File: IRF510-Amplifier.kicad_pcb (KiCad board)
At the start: 2 copper layers, 144.8 x 72.8 mm, 39 parts, among them J1 Jack-DC, J2 BNC, J3 BNC, Q1 2N3904-SMD, Q2 2SC5706, Q4 IRF510, T1 T37-6 15T:7T, U6 MCP1703A-2502_SOT223

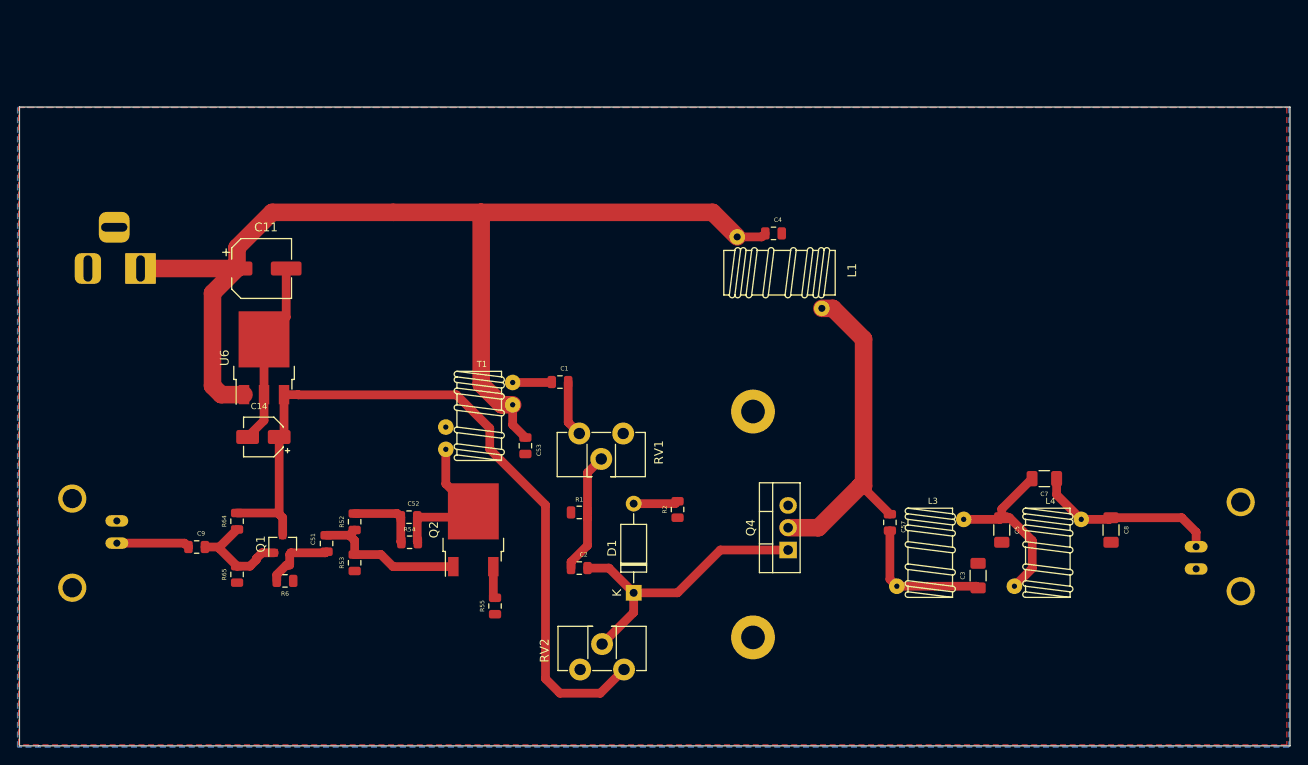
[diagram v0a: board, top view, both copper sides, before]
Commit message: reorg
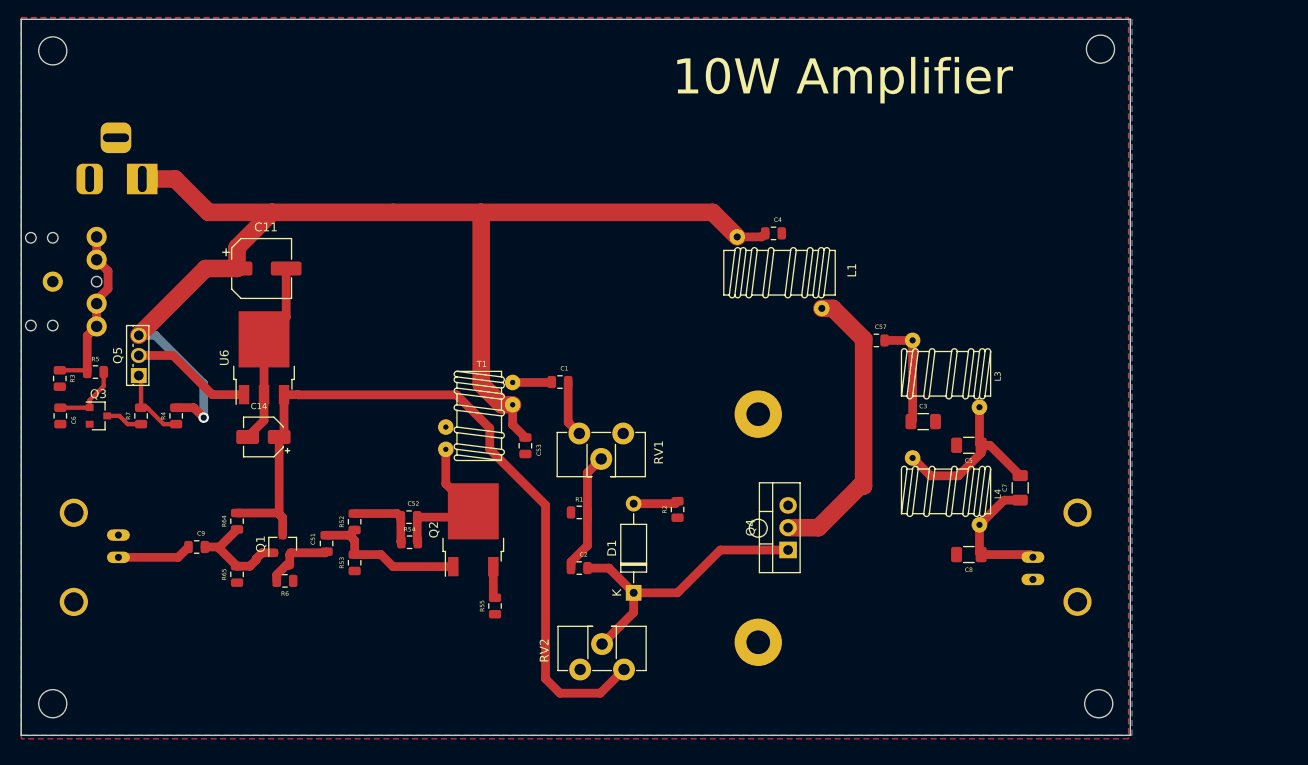
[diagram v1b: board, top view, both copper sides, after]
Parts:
- removed the   at (159.0, 90.2)
- removed the   at (159.0, 64.5)
- added  : , MountingHole:MountingHole_3.2mm_M3, F.Cu at (79.2, 97.8)
- added  : , MountingHole:MountingHole_3.2mm_M3, F.Cu at (198.4, 97.8)
- added  : , MountingHole:MountingHole_3.2mm_M3, F.Cu at (198.6, 23.2)
- added  : , MountingHole:MountingHole_3.2mm_M3, F.Cu at (79.2, 23.4)
- added  : , Xenir:Heatsink_Mounting_25mm, F.Cu at (159.6, 64.8)
- added C6: .1uF, Xenir:Capacitor 0805, F.Cu at (82.6, 65.0)
- added J4: Audio_Jack, Xenir:Audio_Jack, B.Cu at (81.2, 58.2)
- added Q3: BS170F, Package_TO_SOT_SMD:SOT-23, F.Cu at (84.4, 65.0)
- added Q5: IRFU9024, Package_TO_SOT_THT:TO-251-3_Vertical, F.Cu at (89.0, 60.4)
- added R3: 10k, Xenir:Resistor 0805, F.Cu at (77.5, 60.7)
- added R4: 10k, Xenir:Resistor 0805, F.Cu at (95.8, 65.0)
- added R5: 1.5k, Xenir:Resistor 0805, F.Cu at (84.1, 62.5)
- added R7: 10k, Xenir:Resistor 0805, F.Cu at (91.8, 65.0)
- moved C57 23.6 mm to (173.1, 53.9), turned to 0 degrees
- moved C3 20.2 mm to (178.4, 63.4), turned to 0 degrees
- moved C8 19.1 mm to (183.6, 83.0), turned to 180 degrees
- moved J2 18.6 mm to (194.8, 81.0)
- moved L3 16.0 mm to (188.0, 60.2), turned to 270 degrees
- moved J1 10.2 mm to (89.4, 38.0)
- moved C5 9.53 mm to (183.6, 70.6), turned to 180 degrees
- moved C7 5.14 mm to (187.2, 73.2), turned to 90 degrees
- moved L4 4.60 mm to (188.0, 73.6), turned to 270 degrees
- moved J3 1.63 mm to (82.8, 81.2)
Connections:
- U6 pad 1: +12V -> Net-(Q5-Pad2)
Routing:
- net Net-(J4-PadRING): track 0.00 -> 20.1 mm
- net +12V: track 123.6 -> 142.3 mm, vias 0 -> 1
- net Net-(Q5-Pad2): track 0.00 -> 13.8 mm
- net Net-(Q5-Pad1): track 0.00 -> 8.55 mm
- net Net-(C6-Pad1): track 0.00 -> 8.06 mm
- net Net-(C7-Pad1): track 21.3 -> 15.3 mm
- net Net-(Q3-Pad3): track 0.00 -> 4.25 mm
- net Net-(C57-Pad1): track 38.2 -> 33.9 mm
- net Net-(C3-Pad1): track 16.0 -> 12.5 mm
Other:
- board size 144.8 x 72.8 mm -> 126.4 x 81.6 mm
- board text added: "10W Amplifier"
